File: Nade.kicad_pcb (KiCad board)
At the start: 4 copper layers, 35 x 35 mm, 45 parts, among them J1 FTSH-107-01-L-DV-K, J2 Conn_01x03_Pin, J3 Extra, J4 BATT, J5 MEM2085-00-115-00-A_REV0.2, Q1 NMOS, Q2 NMOS, SW2 SW_SPDT, SW3 PTS526 SM15 SMTR2 LFS, U1 MP28160GC-Z, U2 INA213AIRSWR, U3 ADXL314WBCPZ-RL, U4 SSM6N7002KFU_LF

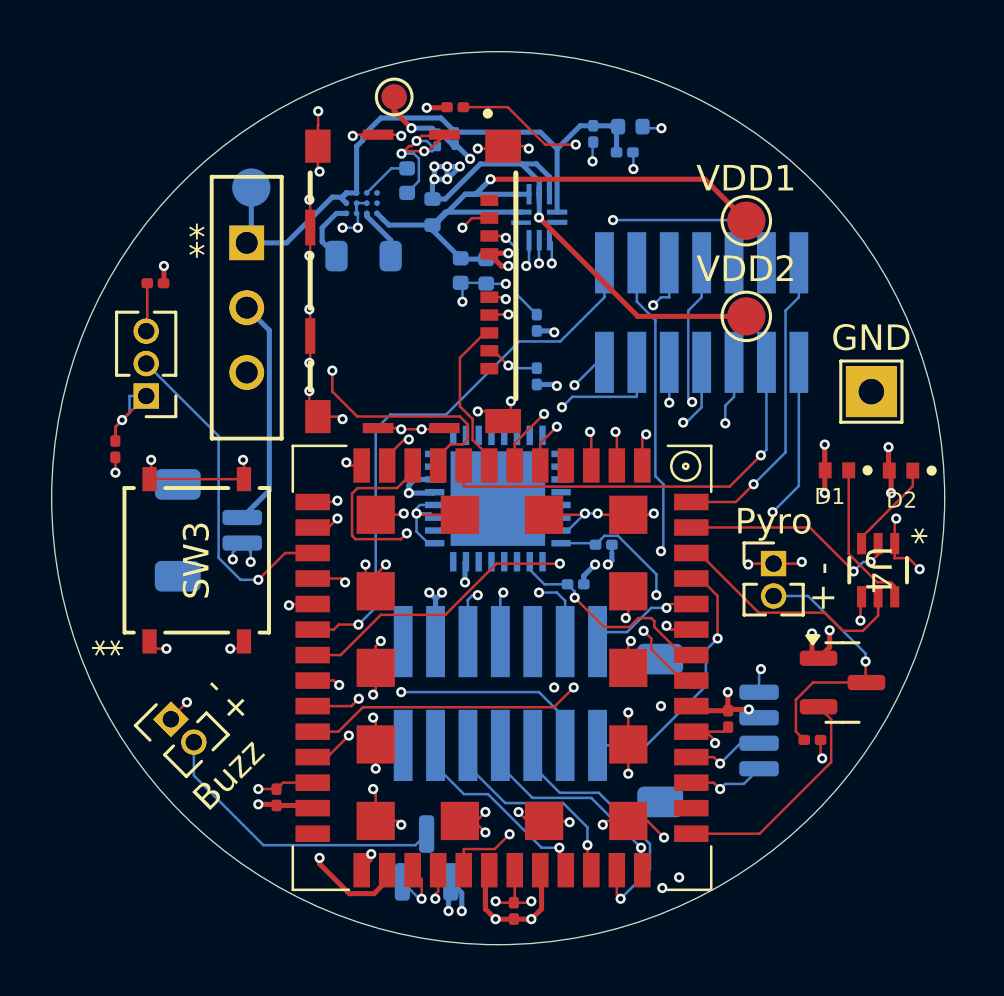
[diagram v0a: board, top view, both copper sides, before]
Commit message: v5
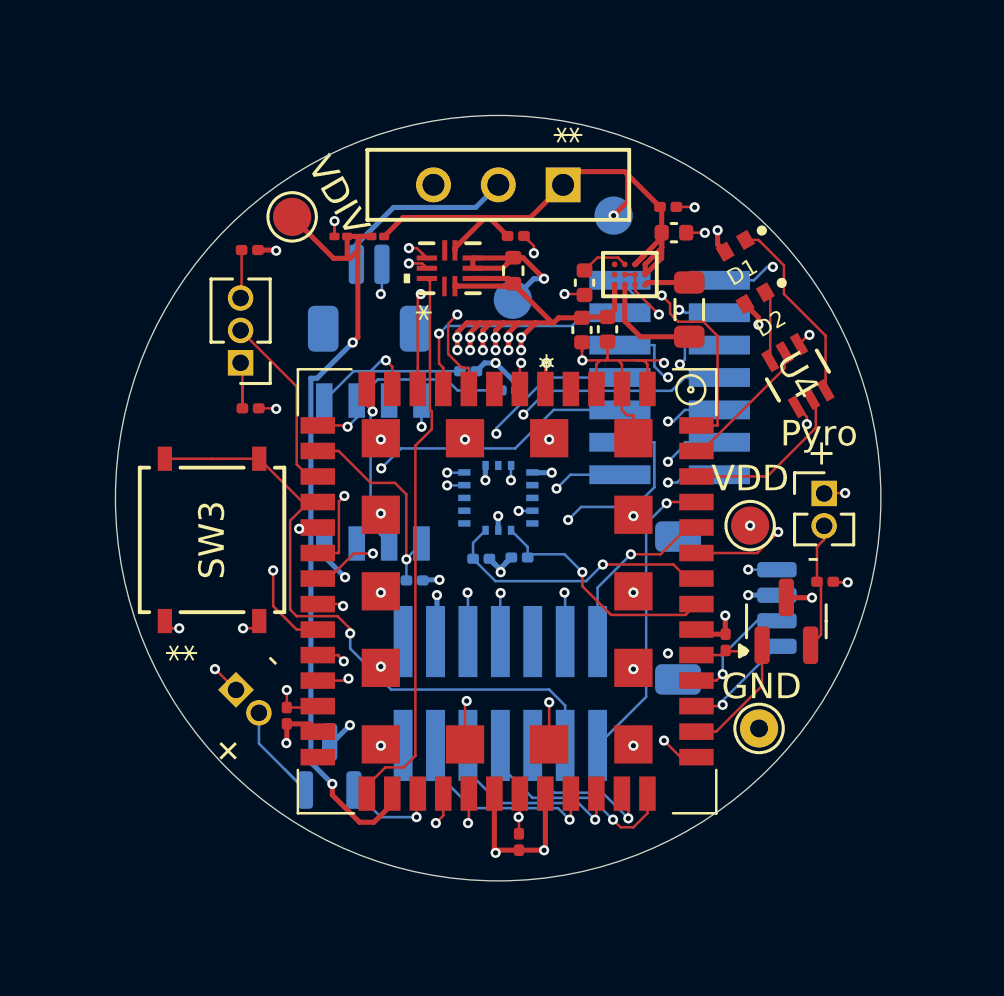
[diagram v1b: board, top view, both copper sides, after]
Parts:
- removed the GND at (144.6, 95.8)
- removed J5: MEM2085-00-115-00-A_REV0.2, footprints:GCT_MEM2085-00-115-00-A_REV0.2
- removed UART: UART, Connector_JST:JST_SH_SM04B-SRSS-TB_1x04-1MP_P1.00mm_Horizontal
- removed VDD1, VDD2: VDD, TestPoint:TestPoint_Pad_D1.5mm
- added GND: GND, TestPoint:TestPoint_THTPad_D1.5mm_Drill0.7mm, F.Cu at (140.2, 109.0)
- added IC1: MB85RS2MTYPNF-G-AWERE2, footprints:SOIC127P600X175-8N, B.Cu at (125.1, 99.0)
- added J7: UART, Connector_JST:JST_SH_SM04B-SRSS-TB_1x04-1MP_P1.00mm_Horizontal, B.Cu at (138.9, 104.3)
- added VDD: VDD, TestPoint:TestPoint_Pad_D1.5mm, F.Cu at (139.9, 101.1)
- added VDD: VDD, TestPoint:TestPoint_Pad_D1.5mm, B.Cu at (130.6, 92.2)
- Buzz, R14: moved to B.Cu
- C10, C5, C6, C7, C8, C9, L1, R10, R11, R12, U1, U2: moved to F.Cu
- R8, R9: value 47 -> 10k
- TP4: footprint TestPoint:TestPoint_Pad_D1.0mm -> TestPoint:TestPoint_Pad_D1.5mm
- U3: value ADXL314WBCPZ-RL -> ADXL373BCCZ-RL7; footprint footprints:LFCSP32_CP-32-17_ADI -> footprints:ADXL373
- moved TP1 14.2 mm to (134.5, 88.9)
- moved L1 12.9 mm to (137.5, 92.6), turned to -90 degrees
- moved SW2 12.6 mm to (132.5, 87.7), turned to -90 degrees
- moved R14 11.3 mm to (130.4, 95.8), turned to 0 degrees
- moved R15 11.2 mm to (126.7, 103.2), turned to 0 degrees
- moved J4 11.1 mm to (124.9, 92.2), turned to 0 degrees
- moved U1 10.9 mm to (135.2, 91.2)
- moved D1 9.66 mm to (139.3, 90.1), turned to -150 degrees
- moved D2 8.85 mm to (140.1, 92.2), turned to -150 degrees
- moved U4 8.25 mm to (141.7, 95.2), turned to -60 degrees
- moved C7 8.02 mm to (133.4, 91.6)
- moved R18 6.22 mm to (142.8, 103.3)
- moved C9 6.20 mm to (134.3, 93.4)
- moved TP4 6.17 mm to (121.9, 89.0)
- moved R9 5.54 mm to (120.3, 96.5), turned to 180 degrees
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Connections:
- C8 pad 1: Net-(U1-OUT) -> VDD
- C9 pad 1: Net-(U1-OUT) -> VDD
- MCU1 pad 27: /PB5 -> Net-(J3-Pin_9)
- MCU1 pad 28: (no net) -> /PB5
- R10 pad 1: VDD -> Net-(R10-Pad1)
- R10 pad 2: Net-(U1-OUT) -> VDD
- R13 pad 1: /PA7 -> /PA4
- R14 pad 1: /PA4 -> /PA6
- R15 pad 1: /PA6 -> /PA7
- U1 pad D3: Net-(U1-OUT) -> VDD
- U2 pad 2: Net-(U1-OUT) -> VDD
- U2 pad 3: Net-(U1-OUT) -> VDD
- U2 pad 4: VDD -> Net-(R10-Pad1)
- U2 pad 5: VDD -> Net-(R10-Pad1)
- U3 pad 1: GND -> VDD
- U3 pad 12: unconnected-(U3-NC-Pad12) -> GND
- U3 pad 13: unconnected-(U3-NC-Pad13) -> GND
- U3 pad 14: unconnected-(U3-NC-Pad14) -> VDD
- U3 pad 16: unconnected-(U3-NC-Pad16) -> GND
- U3 pad 3: GND -> unconnected-(U3-RESERVED-Pad3)
- U3 pad 5: VDD -> unconnected-(U3-RESERVED-Pad5)
- U3 pad 6: VDD -> /PC1
- U3 pad 7: unconnected-(U3-RESERVED-Pad7) -> VDD
- U3 pad 8: unconnected-(U3-NC-Pad8) -> /PC0
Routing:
- net GND: track 117.7 -> 51.2 mm, vias 78 -> 47
- net Net-(J3-Pin_11): track 37.3 -> 9.67 mm, vias 2 -> 1
- net Net-(U1-OUT): track 25.0 -> 0.00 mm, vias 1 -> 0
- net Net-(J3-Pin_9): track 0.00 -> 19.0 mm, vias 0 -> 2
- net /PA4: track 24.2 -> 7.80 mm, vias 3 -> 1
- net Net-(J3-Pin_7): track 35.5 -> 23.5 mm, vias 3 -> 2
- net VDD: track 59.3 -> 49.3 mm
- net Net-(J3-Pin_5): track 29.6 -> 19.6 mm
- net /PA6: track 18.2 -> 8.53 mm, vias 2 -> 1
- net Net-(J3-Pin_3): track 27.7 -> 18.3 mm
- net Net-(J3-Pin_1): track 22.3 -> 14.3 mm, vias 1 -> 2
- net Net-(J3-Pin_8): track 33.9 -> 26.5 mm, vias 3 -> 2
- net Net-(R10-Pad1): track 0.00 -> 6.86 mm, vias 0 -> 1
- net Net-(J8-Pin_2): track 11.7 -> 4.90 mm
- net Net-(J3-Pin_10): track 23.7 -> 17.3 mm
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- added copper zone on In1.Cu, net GND
- added copper zone on In2.Cu, net VDD
- removed copper zone on In2.Cu, net GND
- removed copper zone on In1.Cu, net VDD
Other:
- board size 35 x 35 mm -> 30 x 30 mm
- board text added: "VDIV"
- board text added: "x"
- board text removed: "29"
- board text removed: "30"
- board text removed: "VRAW"
